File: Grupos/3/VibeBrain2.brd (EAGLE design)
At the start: 37 x 18 mm, 39 parts, among them J1 TC2030-IDC, U1 TPS62203DBVR, U2 DRV2605LDGSR, U3 MCP73831T-2ACI/OT

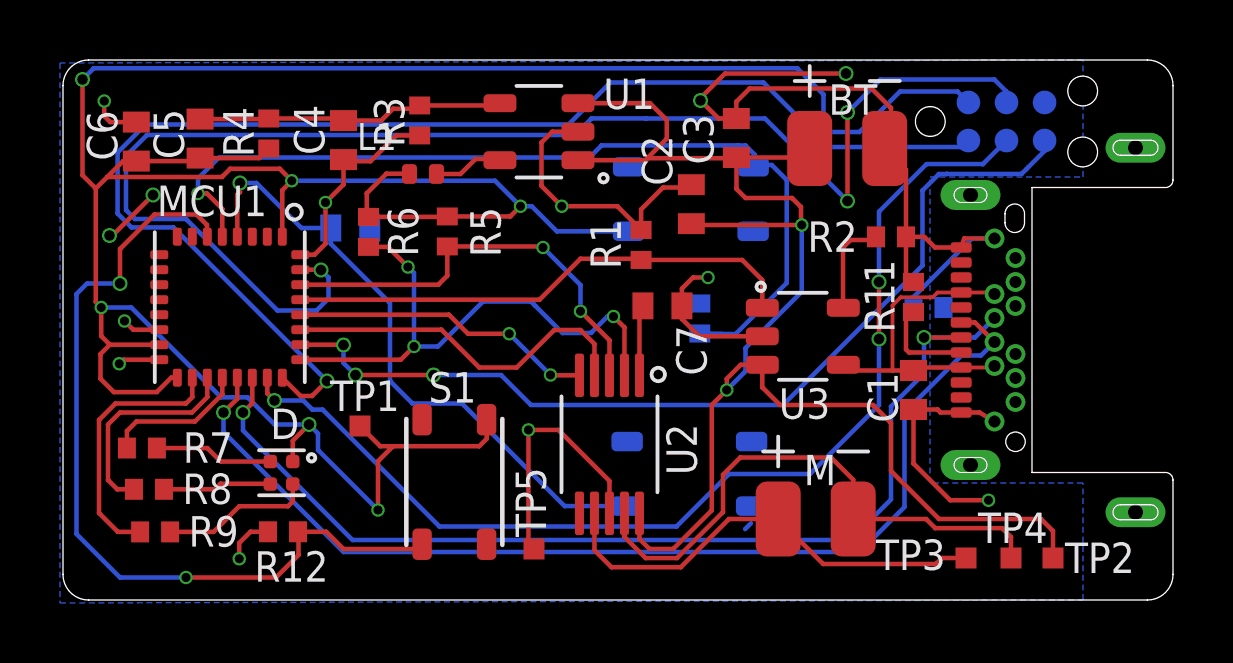
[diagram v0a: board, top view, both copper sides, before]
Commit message: FAltó guardar
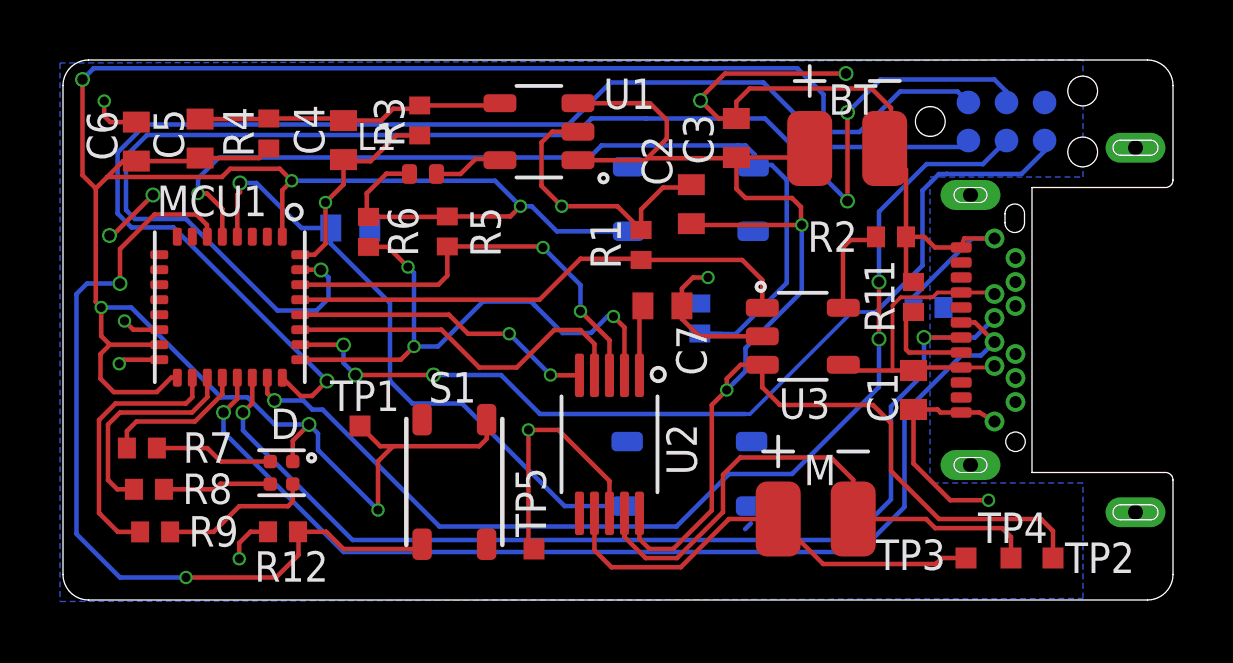
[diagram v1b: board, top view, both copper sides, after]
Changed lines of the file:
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@@
 <polygon width="0.1524" layer="16">
 <vertex x="-0.1" y="17.9"/>
-<vertex x="-0.1" y="-0.1"/>
-<vertex x="34" y="0"/>
+<vertex x="-0.1" y="-0.049853125"/>
+<vertex x="34" y="0.050146875"/>
 <vertex x="34" y="3.9"/>
 <vertex x="28.9" y="3.9"/>
@@
 <wire x1="30.3" y1="12.05" x2="31.05" y2="12.05" width="0.1524" layer="16"/>
 <wire x1="28.35" y1="10.1" x2="30.3" y2="12.05" width="0.1524" layer="16"/>
-<wire x1="22.955" y1="5.28" x2="22.93" y2="2.555" width="0" layer="19" extent="16-16"/>
 </signal>
 <signal name="VDD">
@@
 <wire x1="7.05" y1="6.65" x2="8.00738125" y2="6.65" width="0.1524" layer="16"/>
 <wire x1="8.00738125" y1="6.65" x2="8.31178125" y2="6.3456" width="0.1524" layer="16"/>
-<wire x1="22.2" y1="4.2" x2="24.9" y2="4.2" width="0.1524" layer="16"/>
-<wire x1="24.9" y1="4.2" x2="27.2" y2="6.5" width="0.1524" layer="16"/>
-<wire x1="27.2" y1="6.5" x2="27.2" y2="8.7" width="0.1524" layer="16"/>
+<wire x1="22.2" y1="4.2" x2="24.3" y2="4.2" width="0.1524" layer="16"/>
+<wire x1="24.3" y1="4.2" x2="27.2" y2="7.1" width="0.1524" layer="16"/>
+<wire x1="27.2" y1="7.1" x2="27.2" y2="8.7" width="0.1524" layer="16"/>
 <via x="27.2" y="8.7" extent="1-16" drill="0.35"/>
 <via x="27.2" y="10.6" extent="1-16" drill="0.35"/>
@@
 <contactref element="J1" pad="6"/>
 <wire x1="32.72" y1="15.315" x2="32.72" y2="14.97" width="0.1524" layer="16"/>
-<wire x1="32.72" y1="14.97" x2="32.175" y2="14.425" width="0.1524" layer="16"/>
-<wire x1="32.175" y1="14.425" x2="32.1" y2="14.35" width="0.1524" layer="16"/>
+<wire x1="32.72" y1="14.97" x2="31.9532" y2="14.2032" width="0.1524" layer="16"/>
 <wire x1="29.458725" y1="14.2032" x2="29.455525" y2="14.2" width="0.1524" layer="16"/>
 <wire x1="29.455525" y1="14.2" x2="29.2" y2="14.2" width="0.1524" layer="16"/>
-<wire x1="32.1" y1="14.35" x2="31.9532" y2="14.2032" width="0.1524" layer="16"/>
 <wire x1="31.9532" y1="14.2032" x2="29.458725" y2="14.2032" width="0.1524" layer="16"/>
 <wire x1="29.2" y1="14.2" x2="28.65" y2="13.65" width="0.1524" layer="16"/>
 <wire x1="28.65" y1="13.65" x2="28.65" y2="11.15" width="0.1524" layer="16"/>
-<wire x1="28.65" y1="11.15" x2="24" y2="6.5" width="0.1524" layer="16"/>
-<wire x1="24" y1="6.5" x2="15.6" y2="6.5" width="0.1524" layer="16"/>
-<wire x1="15.6" y1="6.5" x2="14.6" y2="7.5" width="0.1524" layer="16"/>
+<wire x1="28.65" y1="11.15" x2="27.1" y2="9.6" width="0.1524" layer="16"/>
+<wire x1="22.75" y1="6.2" x2="15.9" y2="6.2" width="0.1524" layer="16"/>
+<wire x1="15.9" y1="6.2" x2="14.6" y2="7.5" width="0.1524" layer="16"/>
 <wire x1="14.6" y1="7.5" x2="12.35" y2="7.5" width="0.1524" layer="16"/>
 <via x="12.35" y="7.5" extent="1-16" drill="0.35"/>
@@
 <wire x1="7.91" y1="8.51" x2="9.34" y2="8.51" width="0.1524" layer="1"/>
 <wire x1="9.34" y1="8.51" x2="9.35" y2="8.5" width="0.1524" layer="1"/>
+<wire x1="27.1" y1="9.6" x2="26.3" y2="9.6" width="0.127" layer="16"/>
+<wire x1="22.9" y1="6.2" x2="22.75" y2="6.2" width="0.127" layer="16"/>
+<wire x1="26.3" y1="9.6" x2="22.9" y2="6.2" width="0.127" layer="16"/>
 </signal>
 <signal name="N$19">
